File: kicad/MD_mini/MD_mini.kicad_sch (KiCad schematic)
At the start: 49 parts, among them J1 Conn_01x02_Pin, J2 Conn_01x03_Pin, J3 Conn_01x02_Pin, J4 Conn_01x02_Pin, J6 Conn_02x03_Odd_Even, U1 IRS2003, U2 SCM3723ASA, U3 IRS2003, U4 ACS711xEXLT-15AB, U7 IRS2003, U8 IRS2003, U9 SCM3723ASA

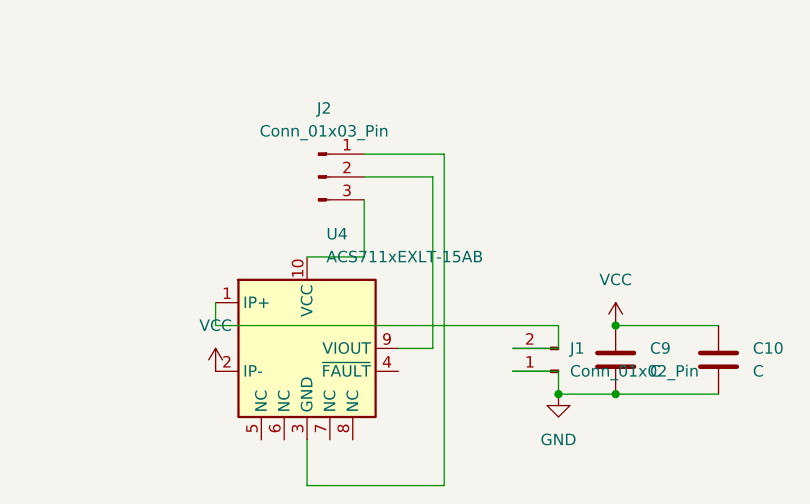
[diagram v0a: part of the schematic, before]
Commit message: a
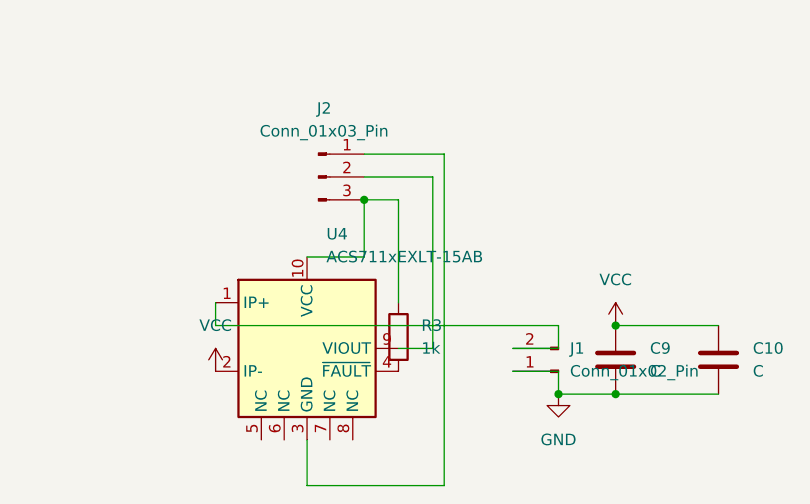
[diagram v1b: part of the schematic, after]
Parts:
- added R3: 1k, symbol Device:R
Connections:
- net at J2.3 (Pin_3), U4.10 (VCC): now also R3.1
- net at U4.4 (~{FAULT}): now also R3.2
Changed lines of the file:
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@@
 	)
 	(junction
+		(at 59.69 148.59)
+		(diameter 0)
+		(color 0 0 0 0)
+	)
+	(junction
 		(at 236.22 105.41)
 		(diameter 0)
@@
 	(wire
 		(pts
+			(xy 63.5 148.59) (xy 63.5 160.02)
+		)
+		(stroke
+			(width 0)
+			(type default)
+		)
+	)
+	(wire
+		(pts
 			(xy 165.1 154.94) (xy 146.05 154.94)
 		)
@@
 	(wire
 		(pts
+			(xy 68.58 143.51) (xy 68.58 180.34)
+		)
+		(stroke
+			(width 0)
+			(type default)
+		)
+	)
+	(wire
+		(pts
 			(xy 226.06 96.52) (xy 226.06 101.6)
 		)
@@
 	(wire
 		(pts
+			(xy 59.69 148.59) (xy 63.5 148.59)
+		)
+		(stroke
+			(width 0)
+			(type default)
+		)
+	)
+	(wire
+		(pts
 			(xy 218.44 57.15) (xy 228.6 57.15)
 		)
@@
 	(wire
 		(pts
-			(xy 68.58 143.51) (xy 68.58 180.34)
-		)
-		(stroke
-			(width 0)
-			(type default)
-		)
-	)
-	(wire
-		(pts
 			(xy 166.37 168.91) (xy 170.18 168.91)
 		)
@@
 					(unit 1)
 				)
+			)
+		)
+	)
+	(symbol
+		(lib_id "Device:R")
+		(at 63.5 163.83 0)
+		(unit 1)
+		(exclude_from_sim no)
+		(in_bom yes)
+		(on_board yes)
+		(dnp no)
+		(fields_autoplaced yes)
+		(property "Reference" "R3"
+			(at 66.04 162.5599 0)
+			(effects
+				(font
+					(size 1.27 1.27)
+				)
+				(justify left)
+			)
+		)
+		(property "Value" "1k"
+			(at 66.04 165.0999 0)
+			(effects
+				(font
+					(size 1.27 1.27)
+				)
+				(justify left)
+			)
+		)
+		(property "Footprint" ""
+			(at 61.722 163.83 90)
+			(effects
+				(font
+					(size 1.27 1.27)
+				)
+				(hide yes)
+			)
+		)
+		(property "Datasheet" "~"
+			(at 63.5 163.83 0)
+			(effects
+				(font
+					(size 1.27 1.27)
+				)
+				(hide yes)
+			)
+		)
+		(property "Description" "Resistor"
+			(at 63.5 163.83 0)
+			(effects
+				(font
+					(size 1.27 1.27)
+				)
+				(hide yes)
+			)
+		)
+		(pin "1"
+		)
+		(pin "2"
+		)
+		(instances
+			(project ""
+				(path "/5b9174b4-8dcf-442c-9b99-056da30be3d5"
+					(reference "R3")
+					(unit 1)
+				)

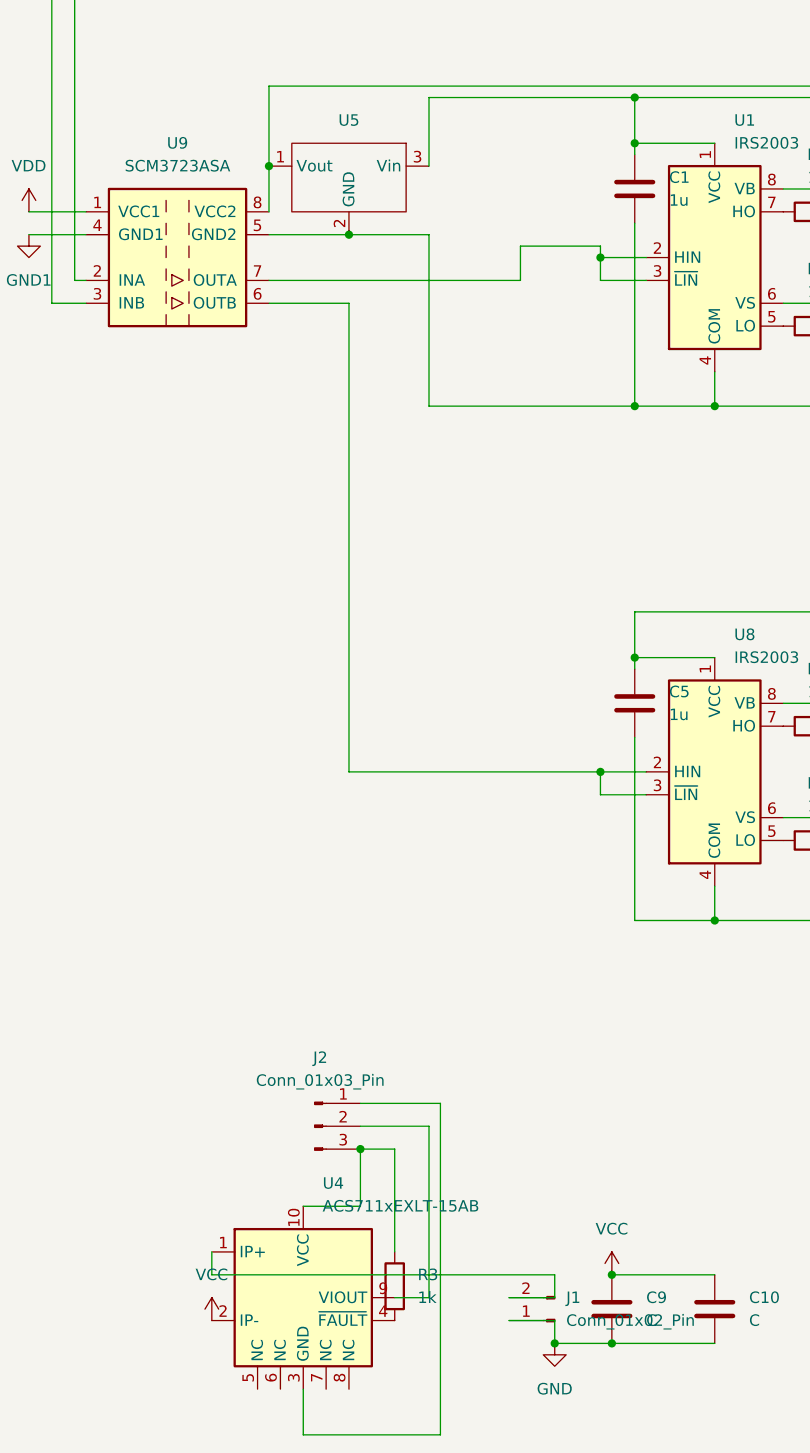
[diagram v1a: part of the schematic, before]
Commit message: a
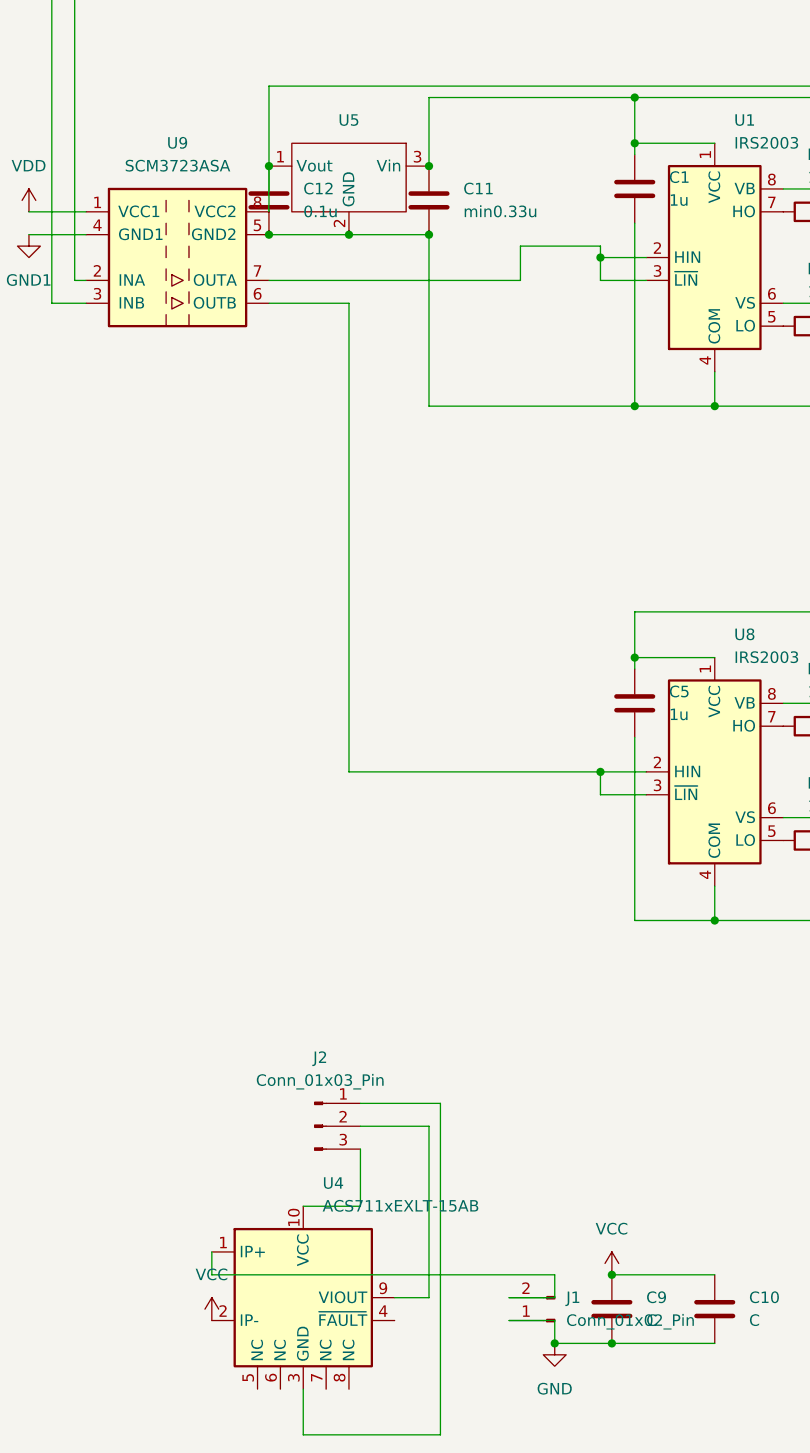
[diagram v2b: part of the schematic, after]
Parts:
- removed R3: 1k, symbol Device:R
- added C11: min0.33u, Capacitor_SMD:C_0603_1608Metric, symbol Device:C
- added C12: 0.1u, Capacitor_SMD:C_0603_1608Metric, symbol Device:C
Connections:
- net GND: now also C11.2, C12.2
- net VCC: now also C11.1
- net at U2.8 (VCC2), U5.1 (Vout), U9.8 (VCC2): now also C12.1
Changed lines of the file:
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@@
 	)
 	(junction
+		(at 49.53 46.99)
+		(diameter 0)
+		(color 0 0 0 0)
+	)
+	(junction
 		(at 219.71 99.06)
 		(diameter 0)
@@
 	)
 	(junction
+		(at 67.31 46.99)
+		(diameter 0)
+		(color 0 0 0 0)
+	)
+	(junction
 		(at 165.1 151.13)
 		(diameter 0)
@@
 	)
 	(junction
-		(at 59.69 148.59)
-		(diameter 0)
-		(color 0 0 0 0)
-	)
-	(junction
 		(at 236.22 105.41)
 		(diameter 0)
@@
 	)
 	(junction
+		(at 67.31 39.37)
+		(diameter 0)
+		(color 0 0 0 0)
+	)
+	(junction
 		(at 87.63 162.56)
 		(diameter 0)
@@
 	(wire
 		(pts
-			(xy 63.5 148.59) (xy 63.5 160.02)
-		)
-		(stroke
-			(width 0)
-			(type default)
-		)
-	)
-	(wire
-		(pts
 			(xy 165.1 154.94) (xy 146.05 154.94)
 		)
@@
 	(wire
 		(pts
-			(xy 59.69 148.59) (xy 63.5 148.59)
-		)
-		(stroke
-			(width 0)
-			(type default)
-		)
-	)
-	(wire
-		(pts
 			(xy 218.44 57.15) (xy 228.6 57.15)
 		)
@@
 	)
 	(symbol
+		(lib_id "Device:C")
+		(at 67.31 43.18 0)
+		(unit 1)
+		(exclude_from_sim no)
+		(in_bom yes)
+		(on_board yes)
+		(dnp no)
+		(fields_autoplaced yes)
+		(property "Reference" "C11"
+			(at 71.12 41.9099 0)
+			(effects
+				(font
+					(size 1.27 1.27)
+				)
+				(justify left)
+			)
+		)
+		(property "Value" "min0.33u"
+			(at 71.12 44.4499 0)
+			(effects
+				(font
+					(size 1.27 1.27)
+				)
+				(justify left)
+			)
+		)
+		(property "Footprint" "Capacitor_SMD:C_0603_1608Metric"
+			(at 68.2752 46.99 0)
+			(effects
+				(font
+					(size 1.27 1.27)
+				)
+				(hide yes)
+			)
+		)
+		(property "Datasheet" "~"
+			(at 67.31 43.18 0)
+			(effects
+				(font
+					(size 1.27 1.27)
+				)
+				(hide yes)
+			)
+		)
+		(property "Description" "Unpolarized capacitor"
+			(at 67.31 43.18 0)
+			(effects
+				(font
+					(size 1.27 1.27)
+				)
+				(hide yes)
+			)
+		)
+		(pin "1"
+		)
+		(pin "2"
+		)
+		(instances
+			(project ""
+				(path "/5b9174b4-8dcf-442c-9b99-056da30be3d5"
+					(reference "C11")
+					(unit 1)
+				)
+			)
+		)
+	)
+	(symbol
 		(lib_id "Device:R")
 		(at 110.49 57.15 90)
@@
 	)
 	(symbol
-		(lib_id "Device:R")
-		(at 63.5 163.83 0)
-		(unit 1)
-		(exclude_from_sim no)
-		(in_bom yes)
-		(on_board yes)
-		(dnp no)
-		(fields_autoplaced yes)
-		(property "Reference" "R3"
-			(at 66.04 162.5599 0)
-			(effects
-				(font
-					(size 1.27 1.27)
-				)
-				(justify left)
-			)
-		)
-		(property "Value" "1k"
-			(at 66.04 165.0999 0)
-			(effects
-				(font
-					(size 1.27 1.27)
-				)
-				(justify left)
-			)
-		)
-		(property "Footprint" ""
-			(at 61.722 163.83 90)
-			(effects
-				(font
-					(size 1.27 1.27)
-				)
-				(hide yes)
-			)
-		)
-		(property "Datasheet" "~"
-			(at 63.5 163.83 0)
-			(effects
-				(font
-					(size 1.27 1.27)
-				)
-				(hide yes)
-			)
-		)
-		(property "Description" "Resistor"
-			(at 63.5 163.83 0)
-			(effects
-				(font
-					(size 1.27 1.27)
-				)
-				(hide yes)
-			)
-		)
-		(pin "1"
-		)
-		(pin "2"
-		)
-		(instances
-			(project ""
-				(path "/5b9174b4-8dcf-442c-9b99-056da30be3d5"
-					(reference "R3")
-					(unit 1)
-				)
-			)
-		)
-	)
-	(symbol
 		(lib_id "Connector:Conn_01x02_Pin")
 		(at 140.97 147.32 0)
@@
 					(unit 1)
 				)
+			)
+		)
+	)
+	(symbol
+		(lib_id "Device:C")
+		(at 49.53 43.18 0)
+		(unit 1)
+		(exclude_from_sim no)
+		(in_bom yes)
+		(on_board yes)
+		(dnp no)
+		(fields_autoplaced yes)
+		(property "Reference" "C12"
+			(at 53.34 41.9099 0)
+			(effects
+				(font
+					(size 1.27 1.27)
+				)
+				(justify left)
+			)
+		)
+		(property "Value" "0.1u"
+			(at 53.34 44.4499 0)
+			(effects
+				(font
+					(size 1.27 1.27)
+				)
+				(justify left)
+			)
+		)
+		(property "Footprint" "Capacitor_SMD:C_0603_1608Metric"
+			(at 50.4952 46.99 0)
+			(effects
+				(font
+					(size 1.27 1.27)
+				)
+				(hide yes)
+			)
+		)
+		(property "Datasheet" "~"
+			(at 49.53 43.18 0)
+			(effects
+				(font
+					(size 1.27 1.27)
+				)
+				(hide yes)
+			)
+		)
+		(property "Description" "Unpolarized capacitor"
+			(at 49.53 43.18 0)
+			(effects
+				(font
+					(size 1.27 1.27)
+				)
+				(hide yes)
+			)
+		)
+		(pin "1"
+		)
+		(pin "2"
+		)
+		(instances
+			(project "MD_mini"
+				(path "/5b9174b4-8dcf-442c-9b99-056da30be3d5"
+					(reference "C12")
+					(unit 1)
+				)
